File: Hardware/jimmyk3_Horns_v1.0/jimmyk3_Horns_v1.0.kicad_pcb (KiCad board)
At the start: 2 copper layers, 17 parts, among them J1 Conn_01x03, J2 Conn_01x02, J3 Conn_01x02, J4 Conn_01x02, Q1 Q_NMOS_GDS

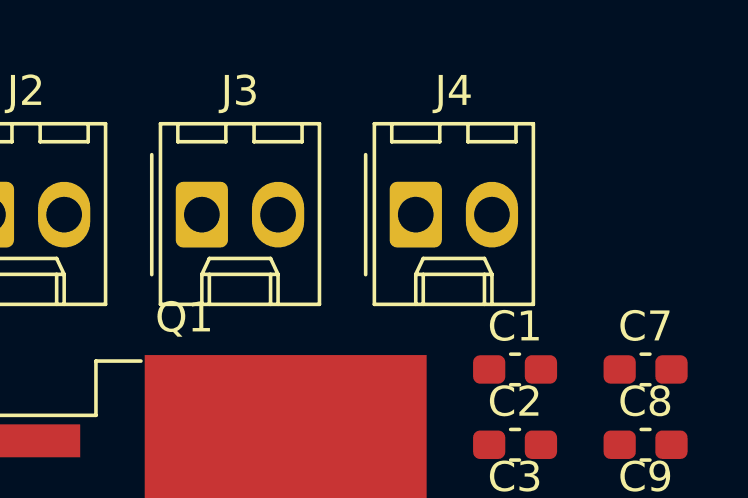
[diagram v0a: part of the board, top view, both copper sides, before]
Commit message: Added layout for hardware project 2
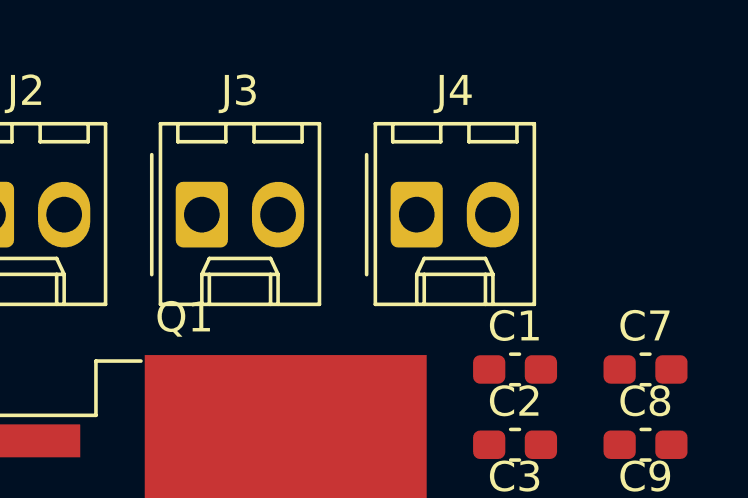
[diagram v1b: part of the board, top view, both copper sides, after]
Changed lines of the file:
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@@
   )
   (footprint "Connector_Molex:Molex_KK-254_AE-6410-02A_1x02_P2.54mm_Vertical" (layer "F.Cu")
-    (at 109.4275 63.8)
+    (at 109.46 63.8)
     (descr "Molex KK-254 Interconnect System, old/engineering part number: AE-6410-02A example for new part number: 22-27-2021, 2 Pins (http://www.molex.com/pdm_docs/sd/022272021_sd.pdf), generated with kicad-footprint-generator")
     (tags "connector Molex KK-254 vertical")
